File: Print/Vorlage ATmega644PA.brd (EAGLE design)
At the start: 80 x 45 mm, 56 parts, among them IC1 ATmega644PA, IC4 ATTINY24/44/84-SSU, Q1 16MHz, X3 87758-3416

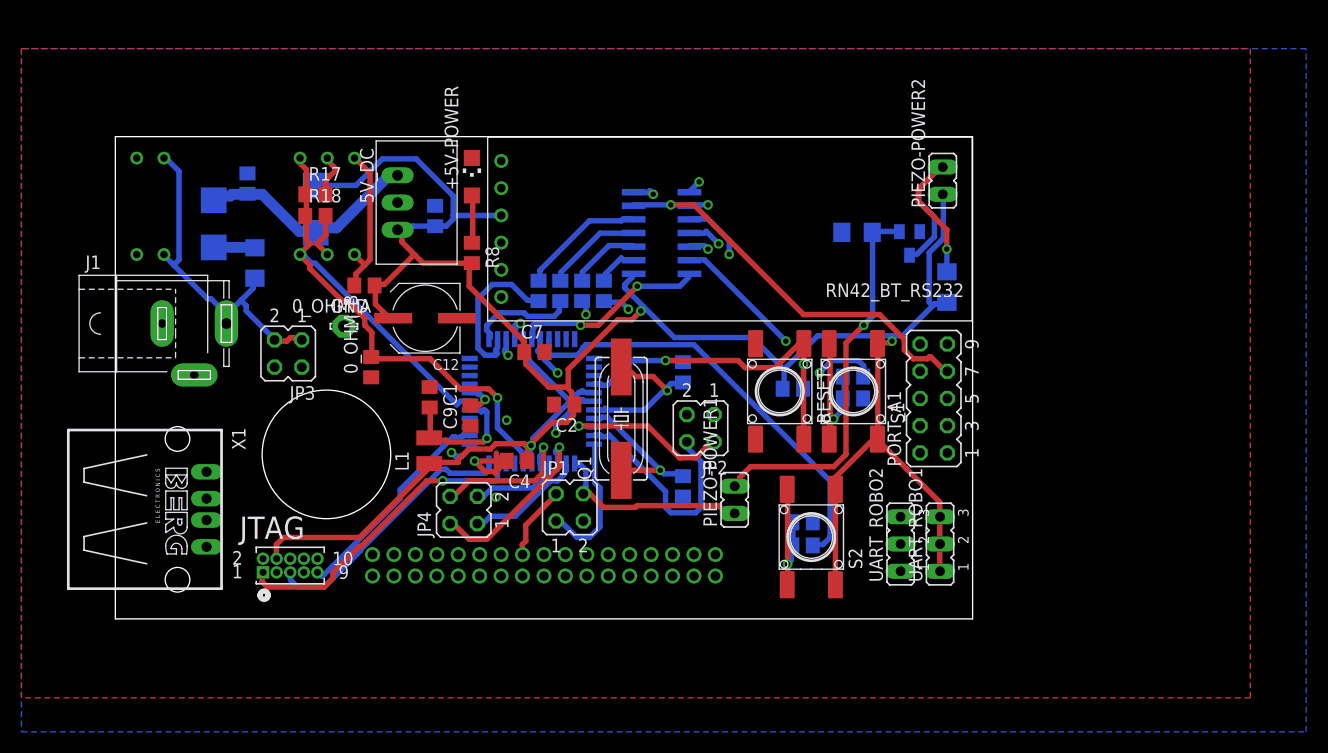
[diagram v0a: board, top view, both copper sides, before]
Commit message: asd
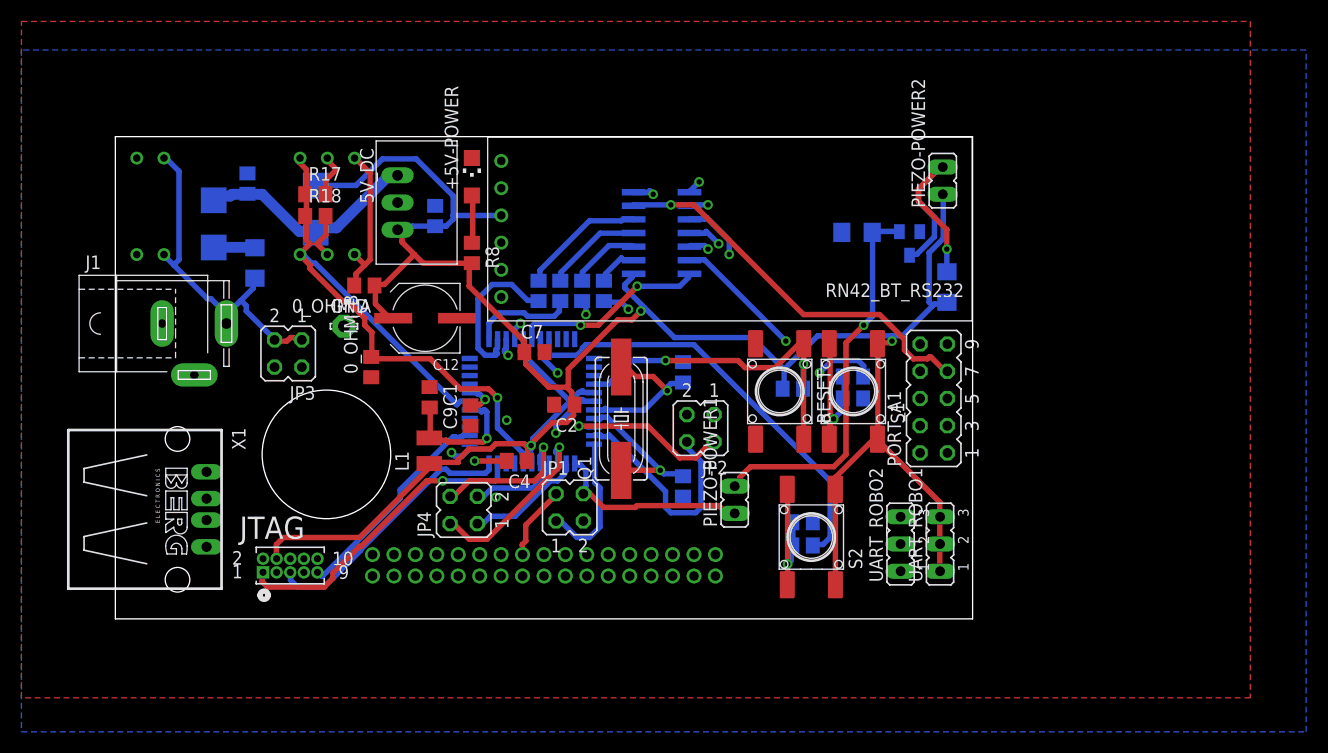
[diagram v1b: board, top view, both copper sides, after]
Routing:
- net GND: track 13.7 -> 8.21 mm
- added copper zone on layer 15, net +5V
